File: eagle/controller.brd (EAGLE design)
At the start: 87.3 x 50.8 mm, 11 parts, among them K1 SRD-05VDC-SL-C, K2 SRD-05VDC-SL-C, K3 SRD-05VDC-SL-C, K4 SRD-05VDC-SL-C

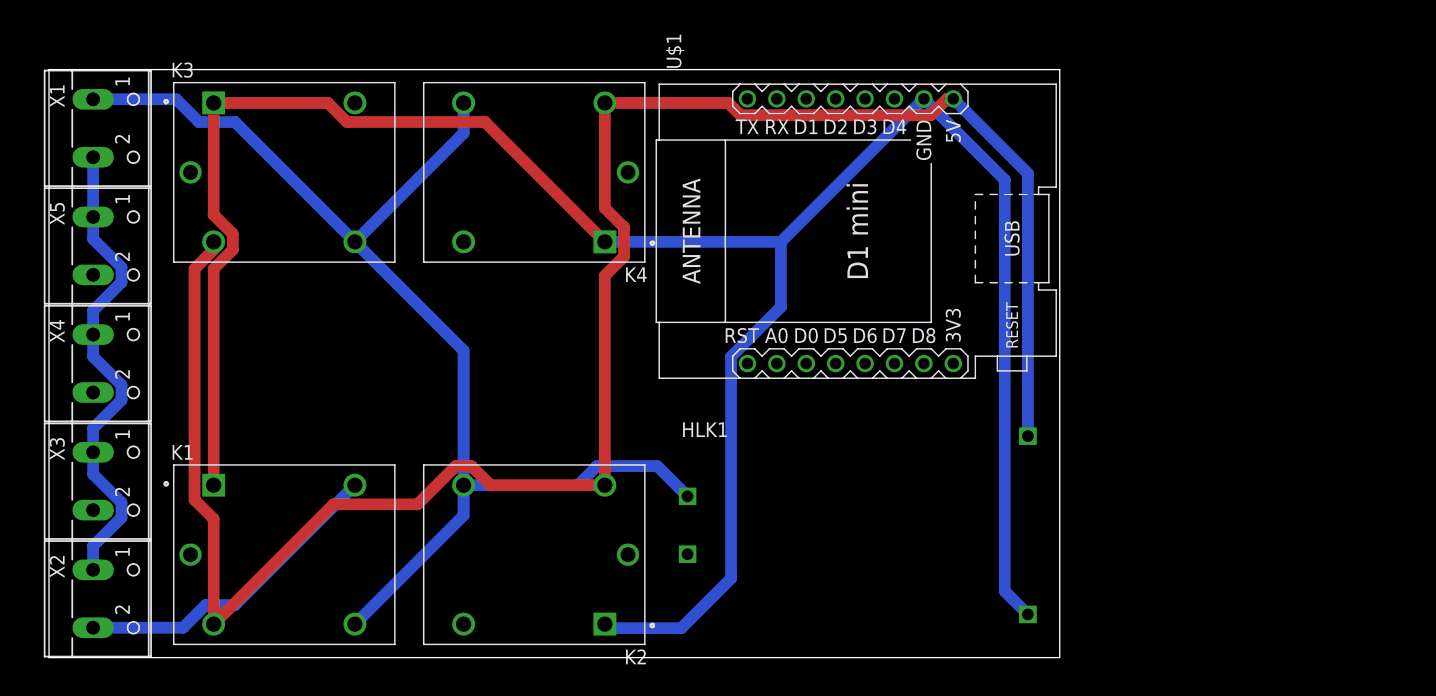
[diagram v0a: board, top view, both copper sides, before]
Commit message: WIP
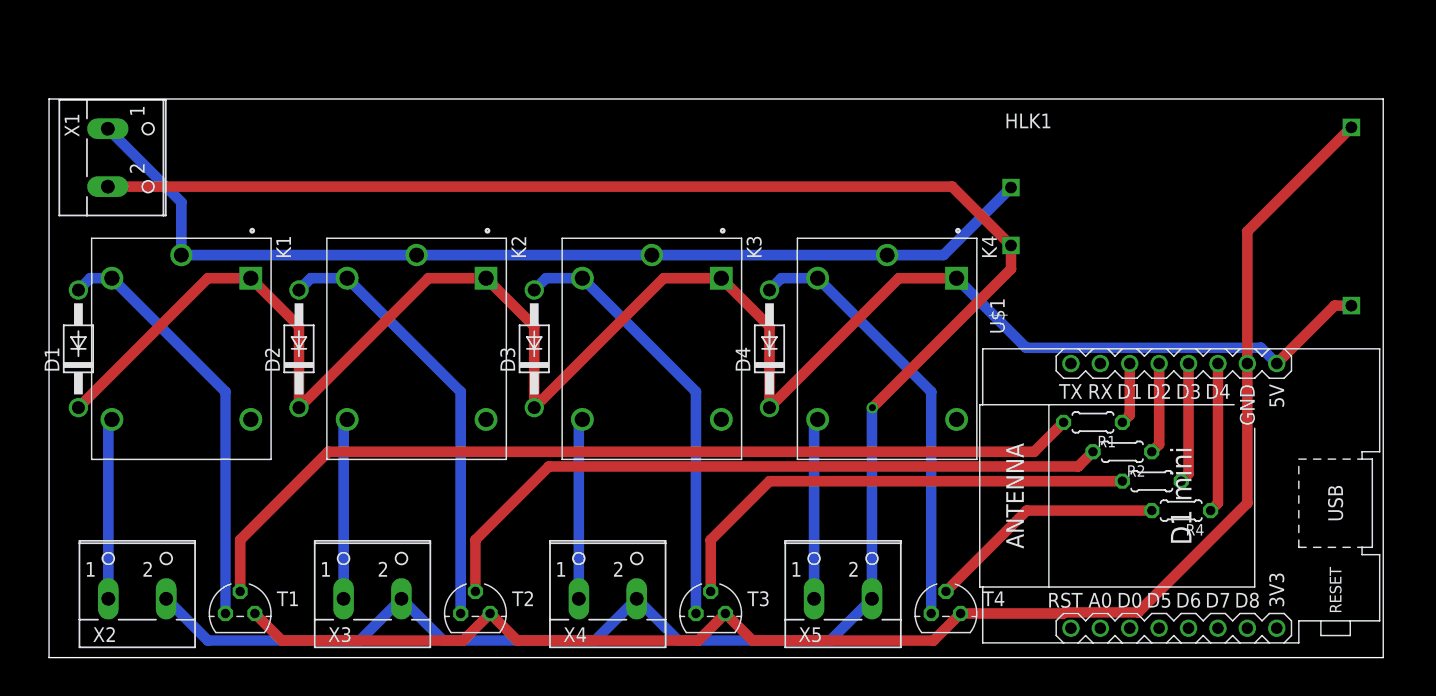
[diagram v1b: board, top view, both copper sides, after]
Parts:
- added D1, D2, D3, D4: 1N4001, tango:DO41-10
- added R1, R2, R3, R4: 1k, rcl:0204/5
- added T1, T2, T3, T4: BC547, transistor:TO92
- X1: value (none) -> VCC
- X2: value (none) -> IN1
- X3: value (none) -> IN2
- X4: value (none) -> IN3
- X5: value (none) -> IN4
- moved X5 69.9 mm to (68.6, 6.35), turned to 0 degrees
- moved X4 47.2 mm to (48.3, 6.35), turned to 0 degrees
- moved HLK1 38.6 mm to (97.8, 38.1)
- moved U$1 36.1 mm to (97.8, 14.0)
- moved K3 35.2 mm to (52.1, 26.7), turned to 270 degrees
- moved K4 34.1 mm to (72.4, 26.7), turned to 270 degrees
- moved X3 24.5 mm to (27.9, 6.35), turned to 0 degrees
- moved K2 20.5 mm to (31.8, 26.7), turned to 270 degrees
- moved K1 19.9 mm to (11.4, 26.7), turned to 270 degrees
- moved X2 2.84 mm to (7.62, 6.35), turned to 0 degrees
- moved X1 2.84 mm to (6.35, 43.2)
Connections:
- removed net N$6: K2.NC, X3.2
- new net 0V: HLK1.P$2, X1.2, X2.2, X3.2, X4.2, X5.2
- new net GND: HLK1.P$3, T1.1, T2.1, T3.1, T4.1, U$1.JP2.7
- new net N$1: D1.A, K1.A2, T1.3
- new net N$10: R4.2, T4.2
- new net N$13: K4.NO, X5.1
- new net N$14: R1.1, U$1.JP2.3
- new net N$15: R2.1, U$1.JP2.4
- new net N$16: R3.1, U$1.JP2.5
- new net N$17: R4.1, U$1.JP2.6
- net +5V: now also D1.C, D2.C, D3.C, D4.C, HLK1.P$4, K1.A1, K2.A1, K3.A1, K4.A1; no longer HLK1.P$3, K1.A2, K2.A2, K3.A2, K4.A2
- net N$11: now also K2.NO, X3.1; no longer HLK1.P$4, K1.A1, K2.A1, K3.A1, K4.A1, U$1.JP2.7
- net N$12: now also K3.NO; no longer HLK1.P$2, X1.2, X2.1, X3.1, X5.1
- net N$2: now also K1.NO, X2.1; no longer K1.COM, U$1.JP2.1, U$1.JP2.2, U$1.JP2.3
- net N$3: now also D2.A, K2.A2, T2.3; no longer K2.COM, U$1.JP2.4
- net N$4: now also D3.A, K3.A2, T3.3; no longer K4.NC, X5.2
- net N$5: now also D4.A, K4.A2, T4.3; no longer K3.NC, X4.2
- net N$7: now also R3.2, T3.2; no longer K1.NC, X2.2
- net N$8: now also R2.2, T2.2; no longer K3.COM, U$1.JP2.5
- net N$9: now also R1.2, T1.2; no longer K4.COM, U$1.JP2.6
- net VCC: now also K1.COM, K2.COM, K3.COM, K4.COM; no longer K1.NO, K2.NO, K3.NO, K4.NO
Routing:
- net 0V: track 0.00 -> 185.8 mm, vias 0 -> 1
- net N$11: track 197.7 -> 15.6 mm
- net GND: track 0.00 -> 131.7 mm
- net N$9: track 0.00 -> 79.8 mm
- net N$8: track 0.00 -> 60.9 mm
- net N$5: track 0.00 -> 37.6 mm
- net N$4: track 0.00 -> 37.6 mm
- net N$3: track 0.00 -> 37.6 mm
- net N$1: track 0.00 -> 36.3 mm
- net N$12: track 41.7 -> 15.6 mm
- net N$10: track 0.00 -> 20.7 mm
- net VCC: track 105.5 -> 87.7 mm
- net N$13: track 0.00 -> 15.6 mm
- net N$2: track 0.00 -> 15.6 mm
- net N$7: track 27.7 -> 42.1 mm
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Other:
- board size 87.3 x 50.8 mm -> 115.2 x 48.2 mm

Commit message: Initial Version
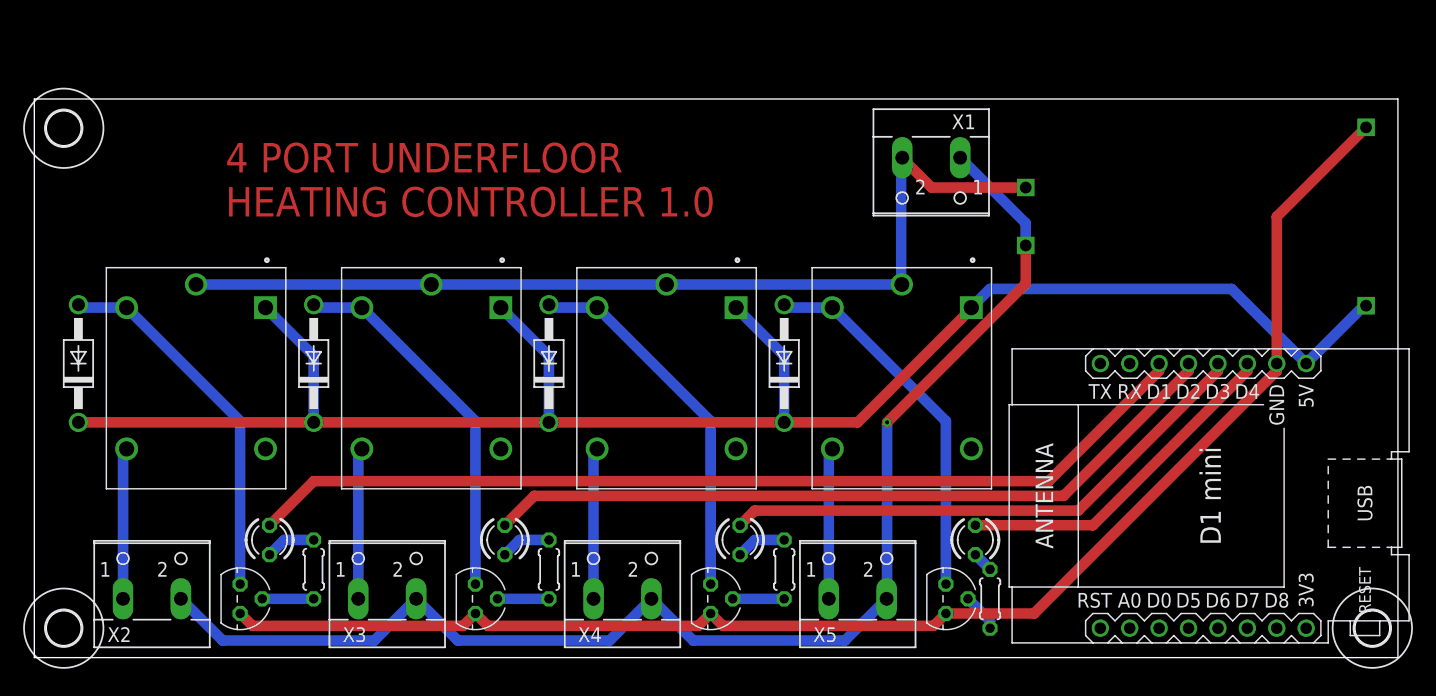
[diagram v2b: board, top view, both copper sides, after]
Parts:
- added LED1, LED2, LED3, LED4: RED, led:LED3MM
- added U$2, U$3, U$4: (no value), holes:3,0
- moved X1 69.9 mm to (76.2, 41.9), turned to 180 degrees
- moved R1 68.5 mm to (22.9, 7.62), turned to 270 degrees
- moved R2 50.6 mm to (43.2, 7.62), turned to 270 degrees
- moved R3 32.7 mm to (63.5, 7.62), turned to 270 degrees
- moved R4 18.2 mm to (81.3, 5.08), turned to 270 degrees
- moved K2 2.84 mm to (33.0, 24.1)
- moved K3 2.84 mm to (53.3, 24.1)
- moved K1 2.84 mm to (12.7, 24.1)
- moved K4 2.84 mm to (73.7, 24.1)
- moved U$1 2.54 mm to (100.3, 14.0)
- moved D3 1.80 mm to (43.2, 25.4)
- moved D4 1.80 mm to (63.5, 25.4)
- moved D2 1.80 mm to (22.9, 25.4)
- moved D1 1.27 mm to (2.54, 25.4)
- moved X4 1.27 mm to (49.5, 6.35)
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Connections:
- new net N$18: LED3.K, R3.1
- new net N$19: LED2.K, R2.1
- new net N$20: LED1.K, R1.1
- new net N$6: LED4.K, R4.1
- net 0V: now also X1.1; no longer X1.2
- net N$14: now also LED1.A; no longer R1.1
- net N$15: now also LED2.A; no longer R2.1
- net N$16: now also LED3.A; no longer R3.1
- net N$17: now also LED4.A; no longer R4.1
- net VCC: now also X1.2; no longer X1.1
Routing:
- net N$14: track 5.34 -> 83.0 mm
- net N$9: track 79.8 -> 4.45 mm
- net 0V: track 185.8 -> 115.6 mm
- net N$15: track 7.88 -> 65.2 mm
- net N$8: track 60.9 -> 4.45 mm
- net N$7: track 42.1 -> 4.45 mm
- net N$16: track 10.4 -> 47.4 mm
- net N$10: track 20.7 -> 3.33 mm
- net N$17: track 13.0 -> 29.7 mm
- net GND: track 131.7 -> 125.1 mm
- net N$5: track 37.6 -> 32.2 mm
- net N$4: track 37.6 -> 32.2 mm
- net N$3: track 37.6 -> 32.2 mm
- net N$19: track 0.00 -> 4.34 mm
- net N$18: track 0.00 -> 4.34 mm
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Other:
- board size 115.2 x 48.2 mm -> 117.8 x 48.2 mm
- board text added: "4 PORT UNDERFLOOR HEATING CONTROLLER 1.0"
